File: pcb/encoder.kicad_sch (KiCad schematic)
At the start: 5 parts, among them J17 Conn_01x04_Pin

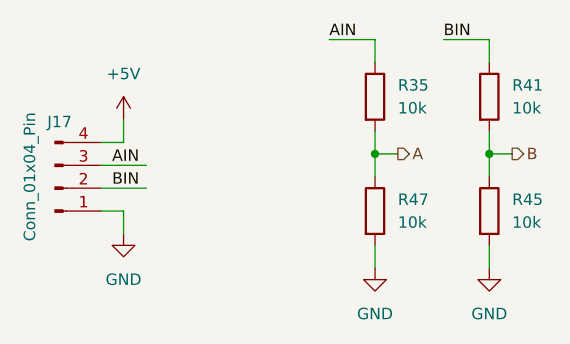
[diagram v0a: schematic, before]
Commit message: Save progress
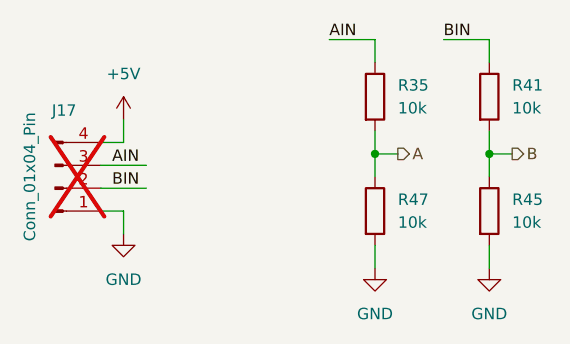
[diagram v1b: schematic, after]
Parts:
- J17: now not fitted
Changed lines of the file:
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@@
 		(in_bom yes)
 		(on_board yes)
-		(dnp no)
+		(dnp yes)
 		(property "Reference" "J17"
-			(at 56.388 51.054 0)
+			(at 56.896 49.784 0)
 			(effects
 				(font
